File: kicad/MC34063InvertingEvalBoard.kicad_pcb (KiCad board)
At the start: 2 copper layers, 49.5 x 49.5 mm, 44 parts, among them P1 CONN_2, P2 CONN_2, U1 MC34063

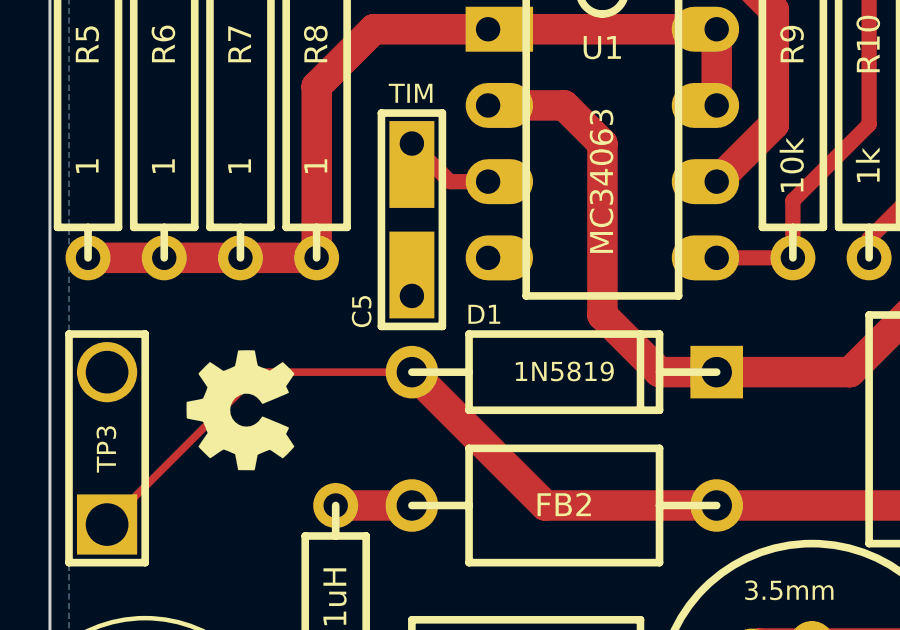
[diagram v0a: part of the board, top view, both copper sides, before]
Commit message: fixing a layout bug
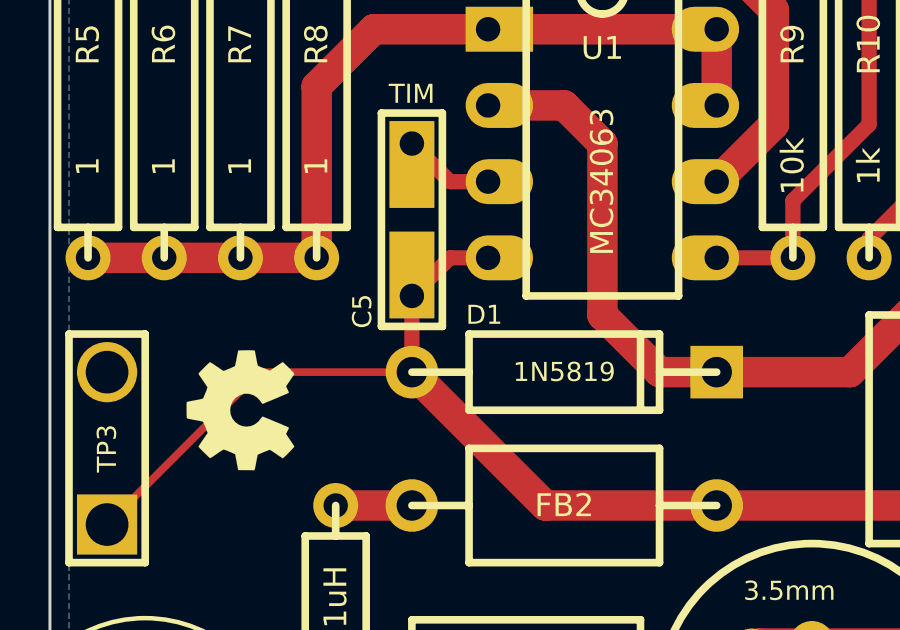
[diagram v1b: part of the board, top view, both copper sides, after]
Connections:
- C5 pad 2: GND -> N-0000014
- U1 pad 4: GND -> N-0000014
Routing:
- net N-0000014: track 65.2 -> 70.8 mm
